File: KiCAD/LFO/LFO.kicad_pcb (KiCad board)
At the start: 2 copper layers, 30 x 100 mm, 16 parts, among them J1 OUT, J2 OUT, J3 Conn_01x03, J4 Conn_01x03, SW1 SW_SPDT, U1 TL072

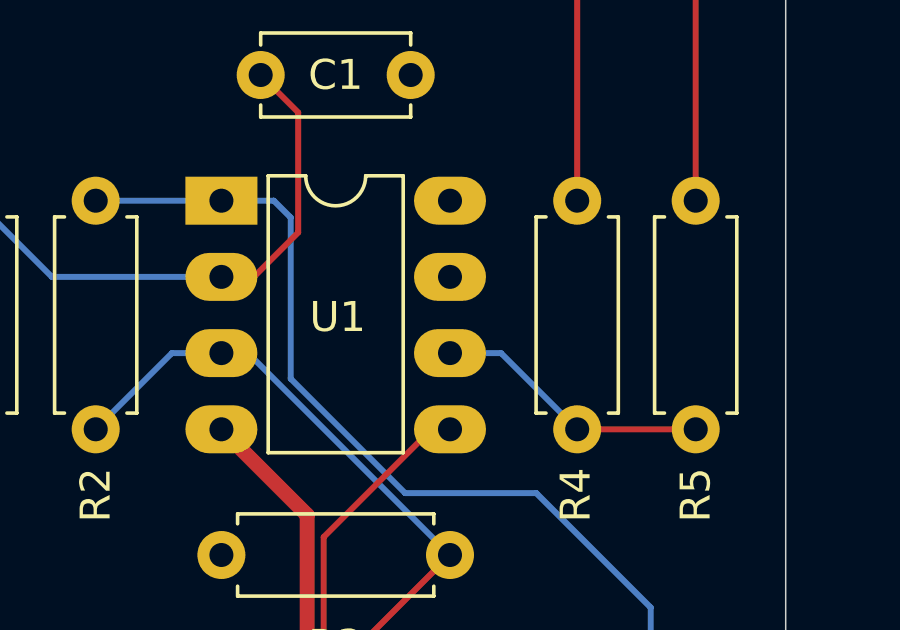
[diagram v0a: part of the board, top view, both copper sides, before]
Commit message: Review
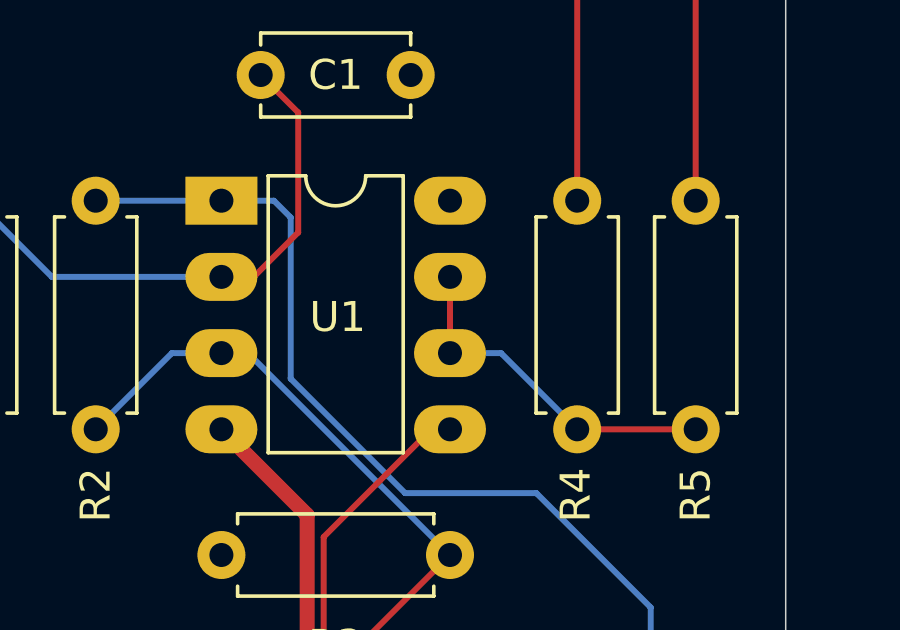
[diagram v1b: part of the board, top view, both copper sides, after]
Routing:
- net Net-(U1B--): track 9.24 -> 11.8 mm
